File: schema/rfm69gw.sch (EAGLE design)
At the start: 18 parts, among them IC1 ESP-12-SMD, IC2 AMS1117-3.3, J1 POWER_JACKPTH, U1 RFM69CW

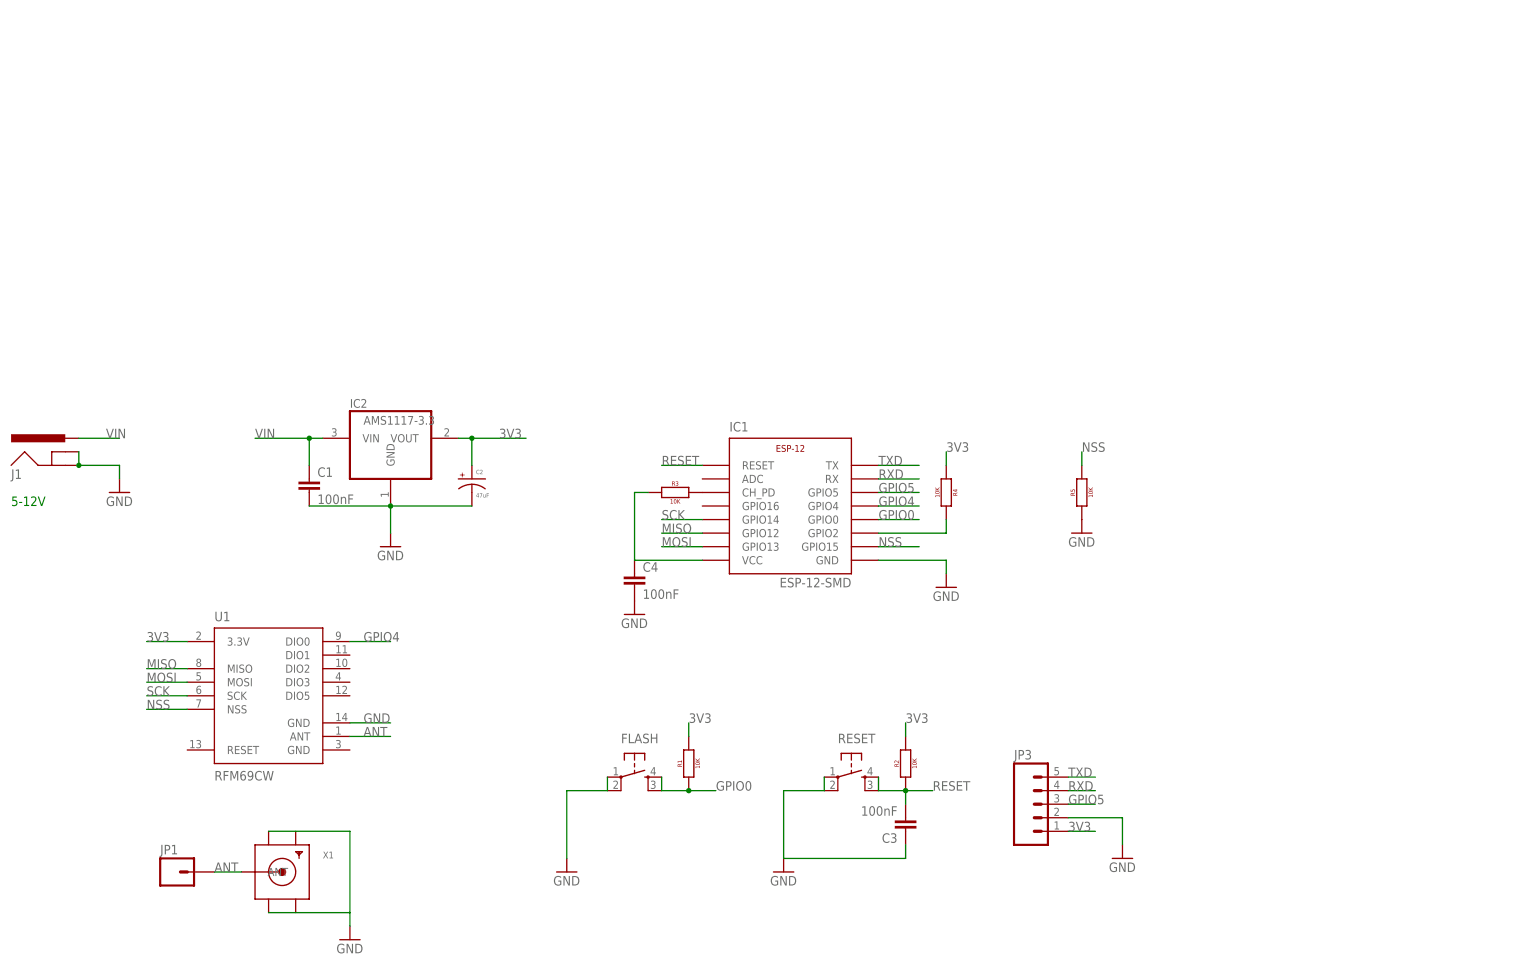
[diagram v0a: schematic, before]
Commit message: Board images
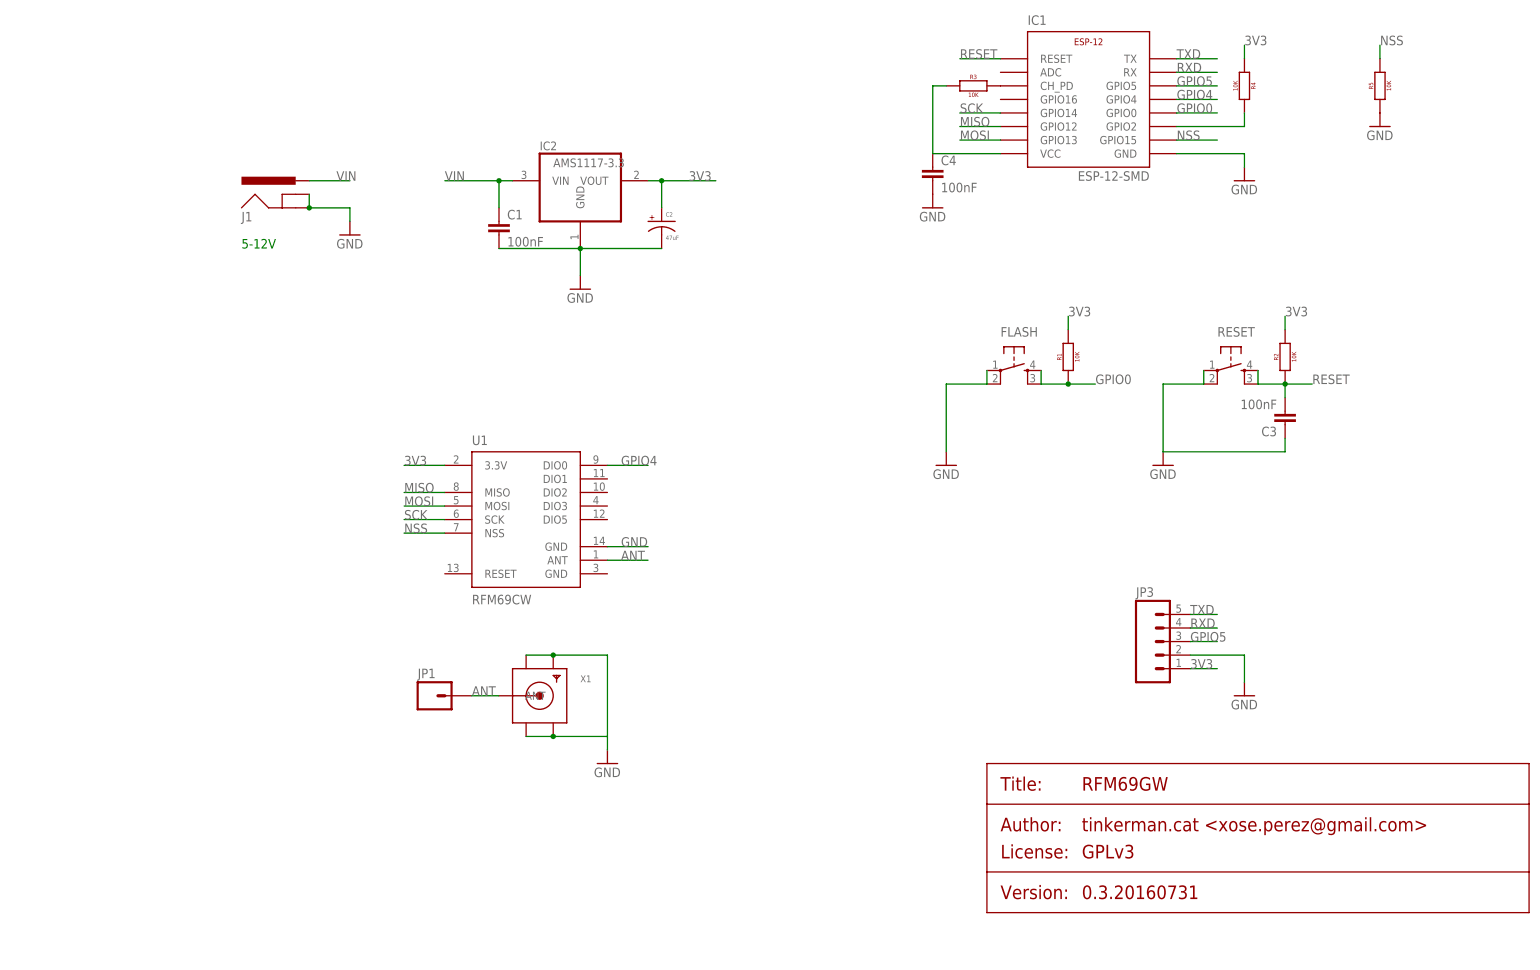
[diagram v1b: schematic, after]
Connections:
- net GND: now also X1.GND2, X1.GND4
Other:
- moved on the sheet: C1, C2, C3, C4, FLASH, IC1, IC2, J1, JP1, JP3, R1, R2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
